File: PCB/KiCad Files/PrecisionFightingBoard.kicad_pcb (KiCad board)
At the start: 2 copper layers, 96.1 x 45.2 mm, 15 parts, among them J1 Conn_01x04_Male, J10 ST01x05, J3 Conn_01x14_Socket, J4 Conn_01x14_Socket, J5 Screw_Terminal_01x03, J6 Conn_02x10_Odd_Even, J7 ST01x05, J8 ST01x05, J9 ST01x05, U1 Teensy4.0

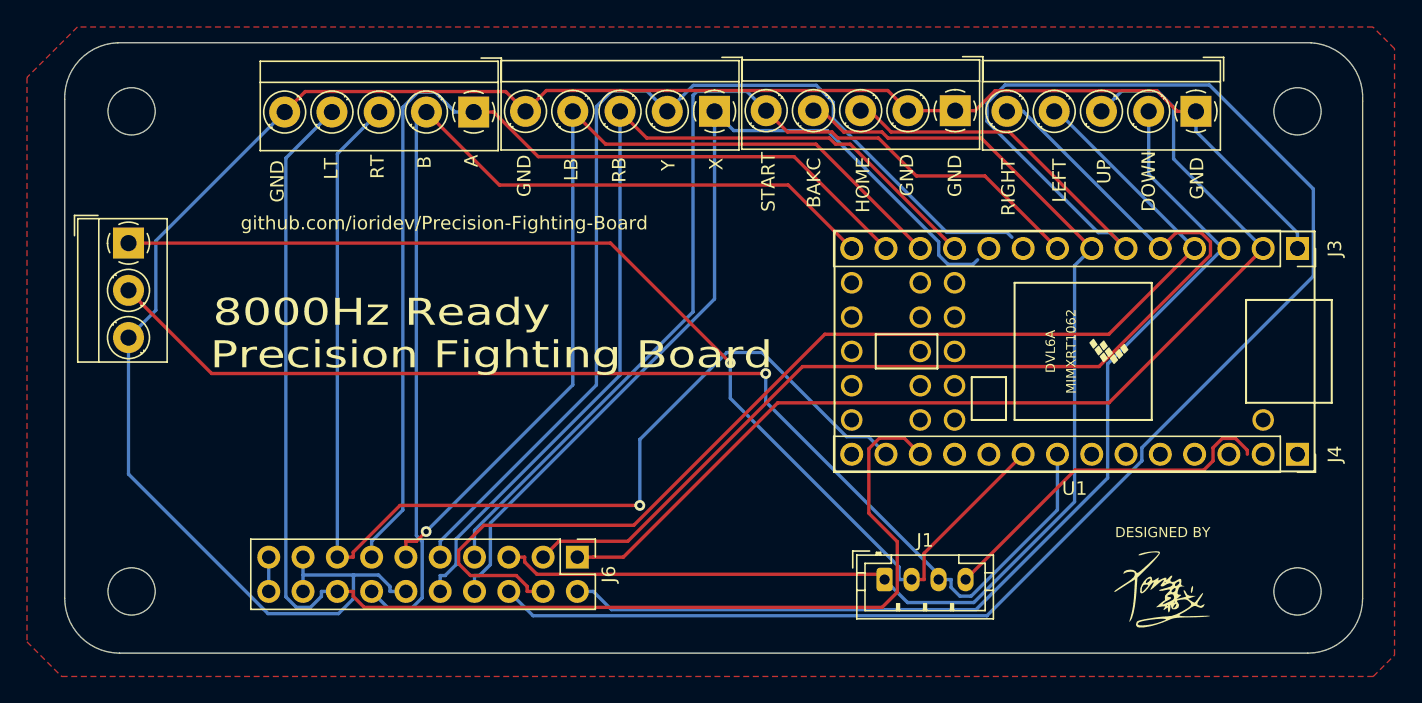
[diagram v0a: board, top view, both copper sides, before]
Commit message: fix pcb
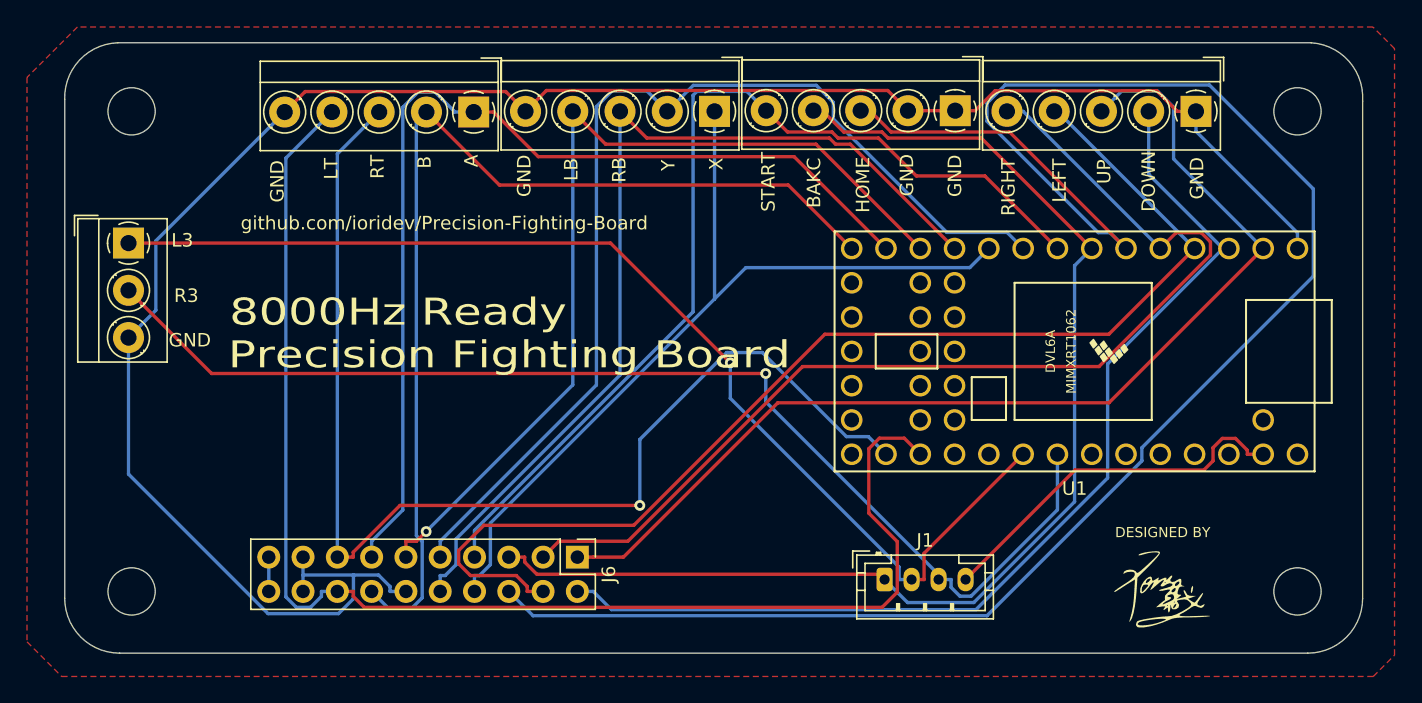
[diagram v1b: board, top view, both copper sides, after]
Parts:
- removed J3, J4: Conn_01x14_Socket, Connector_PinSocket_2.54mm:PinSocket_1x14_P2.54mm_Vertical
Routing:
- net /X: track 68.0 -> 65.0 mm
- net /GND: track 176.6 -> 177.8 mm
- net /Y: track 76.2 -> 77.4 mm
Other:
- board text added: "L3"
- board text added: "R3"
